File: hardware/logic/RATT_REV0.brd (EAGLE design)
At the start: 127 x 76.2 mm, 129 parts, among them IC1 TLP292-4, IC13 MCP73832, IC16 PCA9539PW, IC2 CPC1002N, IC200 TPS2115AIPWRQ1, IC3 CPC1002N, IC300 MAX98357, IC4 CPC1002N, IC5 CPC1002N, IC500 AP2112K-3.3V, J1 4P-2.0, J100 PHOENIX1803426, J2 4P-2.0, J4 4P-2.0, J5 F-1X04-SIP-100-40, J6 4P-2.0, J7 PHOENIX1803484, J8 PHOENIX1803484, J87 RPI-ZERO, Q5 2N7002

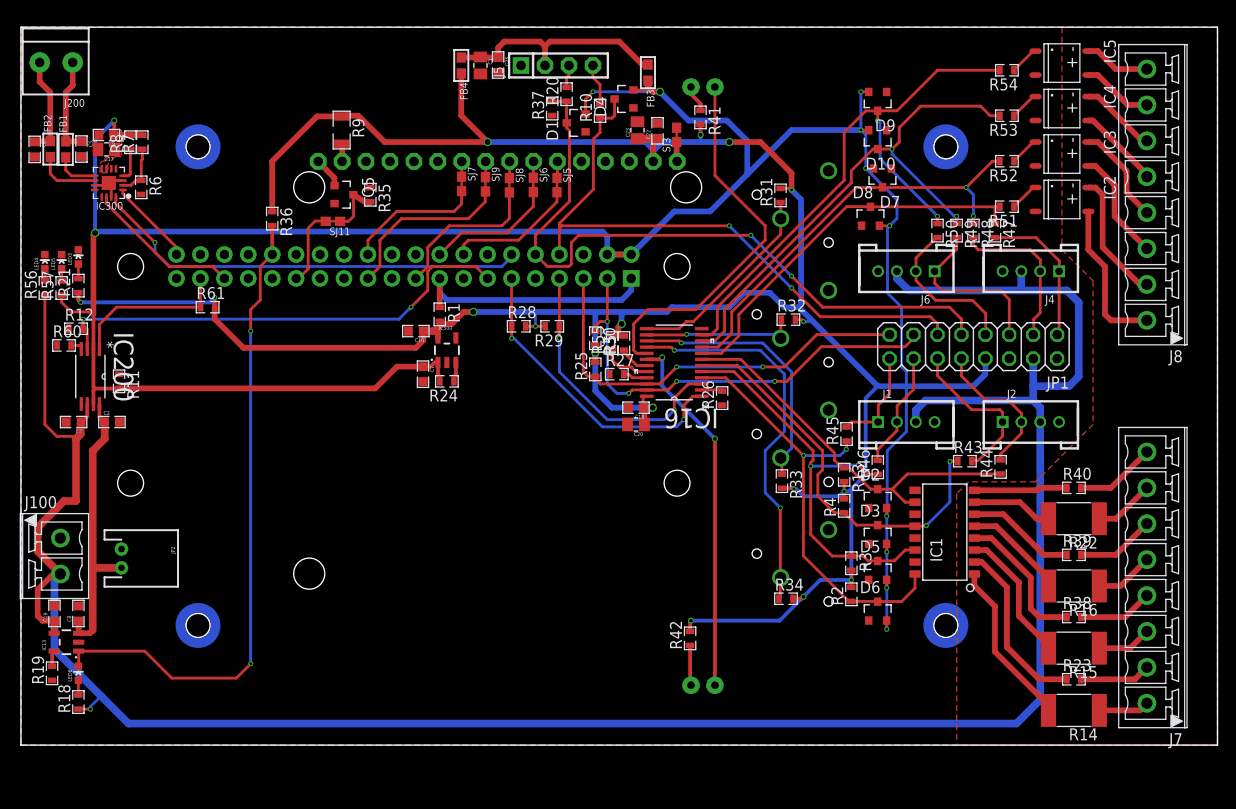
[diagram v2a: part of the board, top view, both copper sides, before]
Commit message: moved stuff for Steve
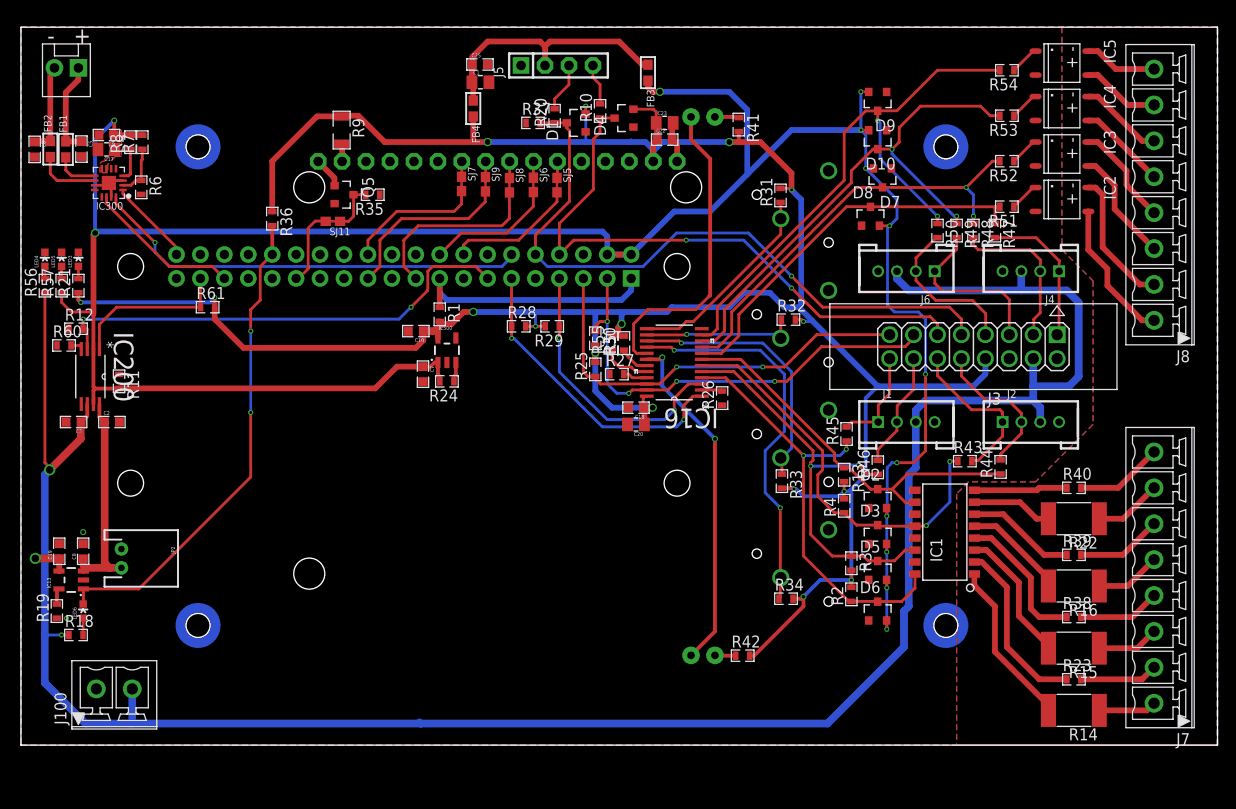
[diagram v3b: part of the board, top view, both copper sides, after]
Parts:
- removed J200: (no value), MakeItLabs:TERMBLOCK_1X2-3.5MM
- removed JP1: (no value), MakeItLabs:2X08
- removed SJ3: JUMPER-PAD-2-NC_BY_TRACE, MakeItLabs:SOLDERJUMPER_10MIL
- added J3: (no value), MakeItLabs:2X08_SHROUD
- added JP4: (no value), MakeItLabs:MOLEX-1X2
- moved J100 16.0 mm to (9.91, 5.33), turned to 0 degrees
- moved R18 7.12 mm to (5.84, 11.7), turned to 0 degrees
- moved C19 6.62 mm to (4.06, 20.6)
- moved C8 6.62 mm to (6.60, 20.6)
- moved LED6 6.62 mm to (6.60, 14.2)
- moved R19 6.62 mm to (3.81, 14.2)
- moved IC13 6.62 mm to (5.33, 17.5)
- moved R42 5.88 mm to (76.6, 9.49), turned to 0 degrees
- moved FB4 4.75 mm to (48.0, 67.6)
- moved R41 4.13 mm to (76.2, 65.9)
- moved LED2 3.18 mm to (72.4, 9.53), turned to 0 degrees
- moved LED1 3.17 mm to (72.4, 66.7), turned to 0 degrees
- moved C23 2.99 mm to (68.3, 66.0), turned to 0 degrees
- moved R20 2.62 mm to (56.6, 66.8)
- moved R37 2.54 mm to (54.4, 66.0), turned to 0 degrees
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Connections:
- removed net N$3: LCD3.1, SJ3.1
- net +3.3V: now also D1.2, D4.2, J3.8; no longer JP1.8
- net +5VB: no longer D1.2, D4.2
- net +5VIN: now also J3.4; no longer JP1.4
- net GND: now also J3.2, J3.6, LCD3.1; no longer JP1.2, JP1.6, SJ3.2
- net I2C_SCL: now also J3.15; no longer JP1.15
- net I2C_SDA: now also J3.13; no longer JP1.13
- net IN0P: now also J3.16; no longer JP1.16
- net IN1P: now also J3.14; no longer JP1.14
- net IN2P: now also J3.12; no longer JP1.12
- net IN3P: now also J3.10; no longer JP1.10
- net N$6: now also JP4.2; no longer J200.1
- net N$7: now also JP4.1; no longer J200.2
- net OUT0P: now also J3.1; no longer JP1.1
- net OUT1P: now also J3.3; no longer JP1.3
- net OUT2P: now also J3.5; no longer JP1.5
- net OUT3P: now also J3.7; no longer JP1.7
- net RFID_RX: now also J3.11; no longer JP1.11
- net RFID_TX: now also J3.9; no longer JP1.9
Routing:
- net CHARGE_STATUS: track 69.1 -> 51.9 mm
- net +5VIN: track 256.3 -> 240.0 mm, vias 1 -> 3
- net V_BATT: track 30.9 -> 23.3 mm
- net LED0: track 40.4 -> 33.5 mm
- net +5VB: track 269.6 -> 263.8 mm, vias 12 -> 13
- net GND: track 4.81 -> 9.24 mm, vias 0 -> 2
- net +3.3V: track 296.3 -> 292.7 mm, vias 17 -> 16
- net LCD_MOSI: track 16.5 -> 19.5 mm
- net N$51: track 24.6 -> 27.5 mm
- net 5V_RFID_TX: track 2.40 -> 5.22 mm
- net N$49: track 4.46 -> 2.21 mm
- net RFID_TX: track 73.2 -> 71.1 mm, vias 2 -> 1
- net LED1: track 38.8 -> 36.7 mm
- net N$3: track 2.08 -> 0.00 mm
- net RFID_RX: track 65.6 -> 63.9 mm
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- added copper zone on layer 16, net N$16
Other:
- board text added: "+"
- board text added: "-"

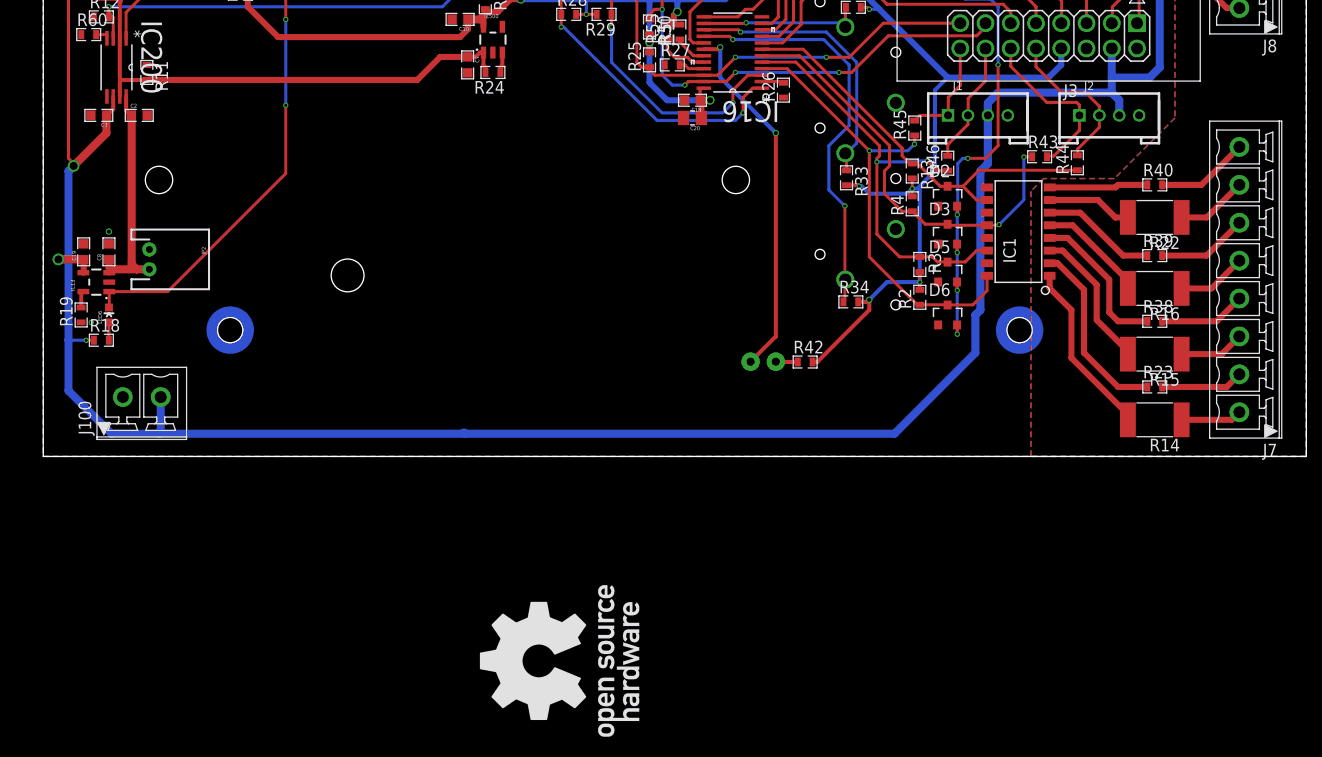
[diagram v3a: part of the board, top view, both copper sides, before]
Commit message: minor tweak
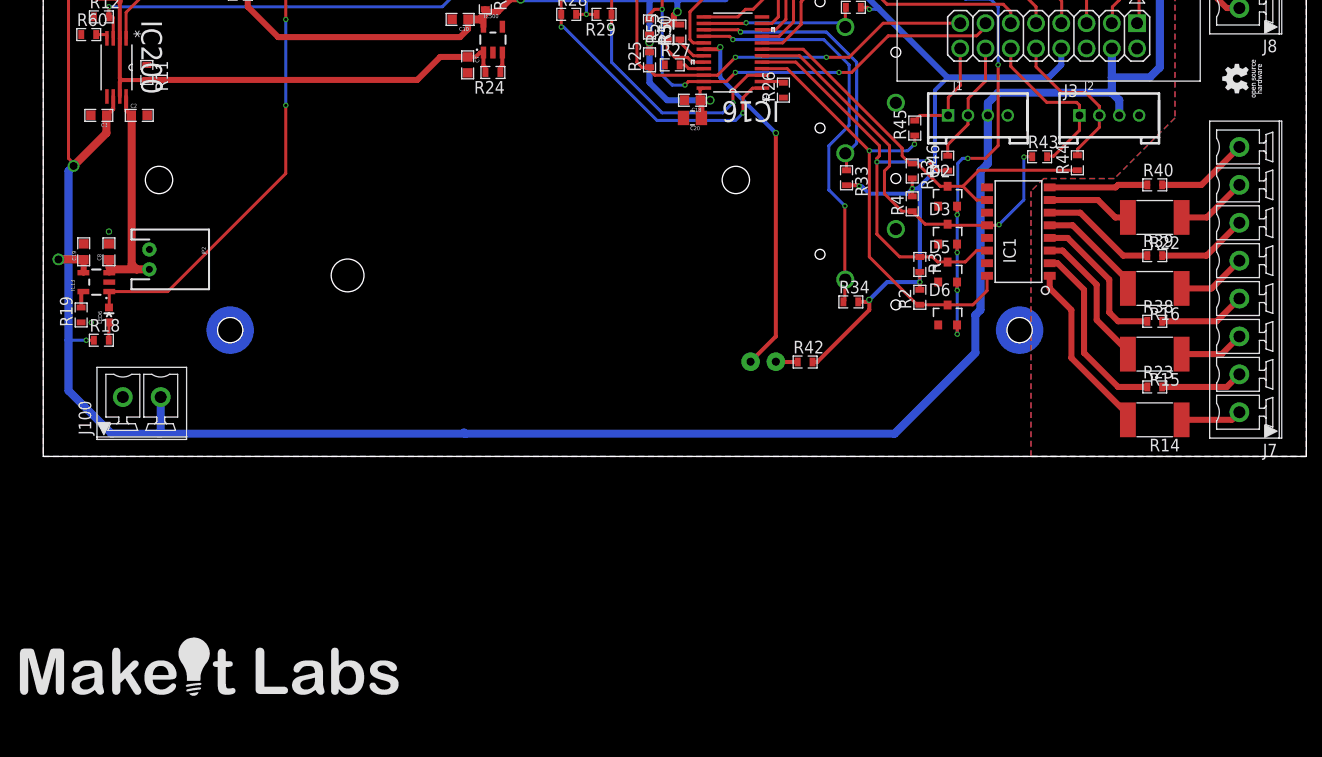
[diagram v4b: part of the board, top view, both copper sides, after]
